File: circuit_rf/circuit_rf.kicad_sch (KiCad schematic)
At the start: 13 parts, among them J18 USB_C_Receptacle_USB2.0, U8 ESP32-C3, U9 SX1279, Y1 16M

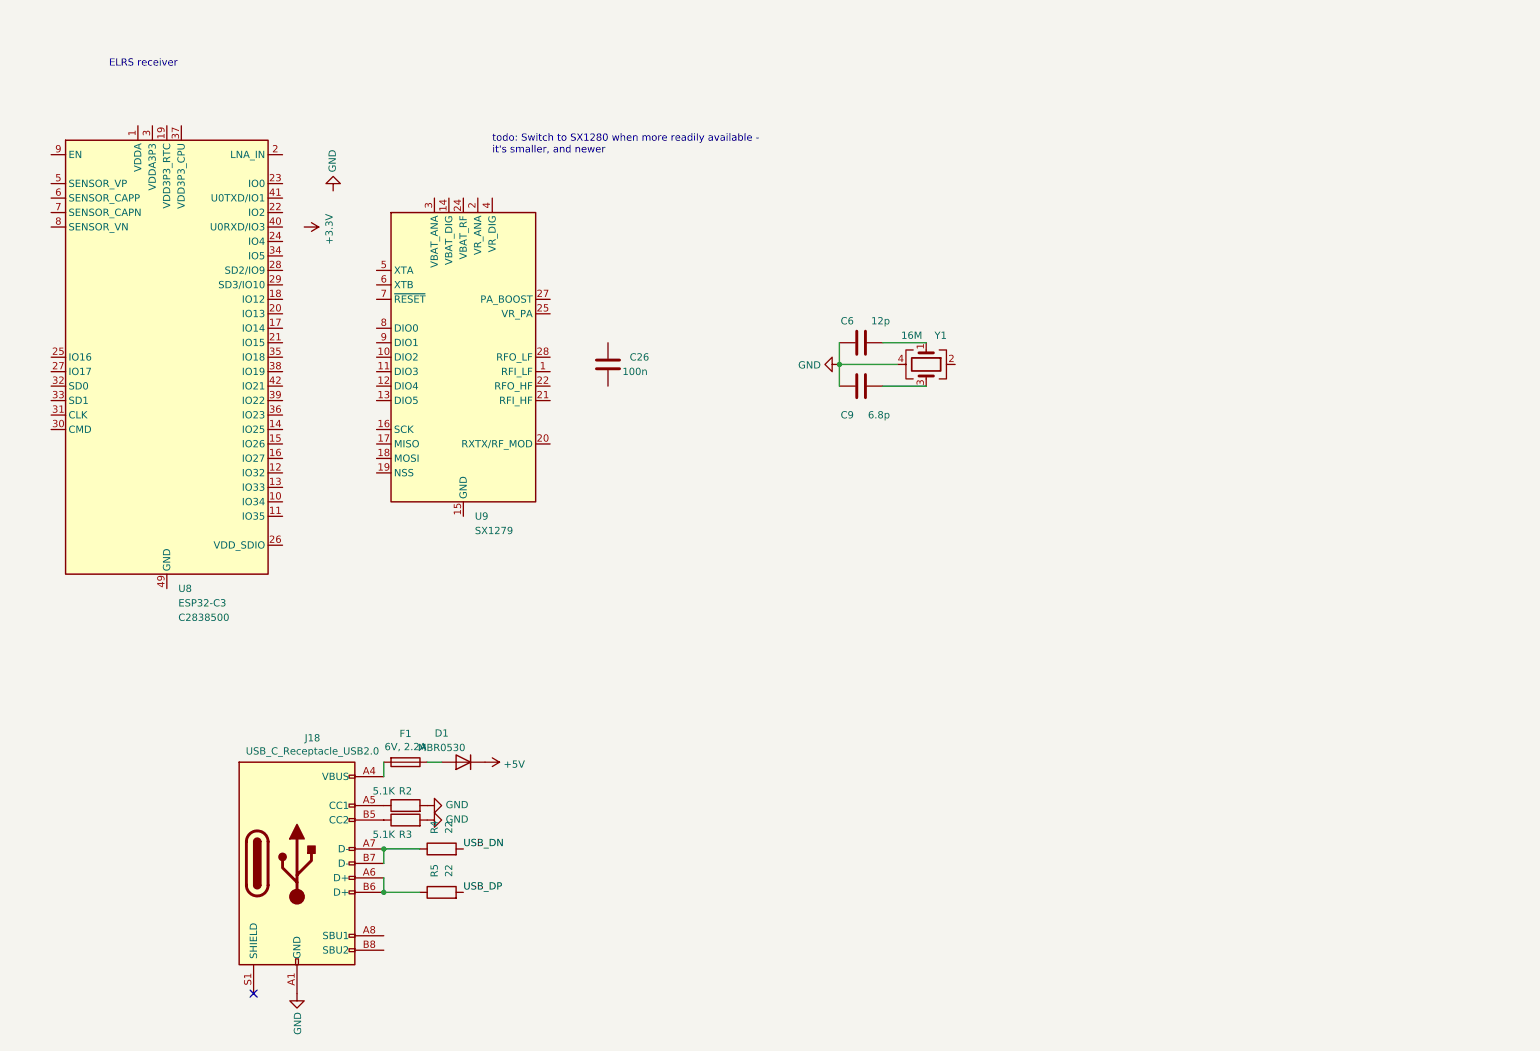
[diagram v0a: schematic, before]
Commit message: Lots of work on schematic, and BF cfg
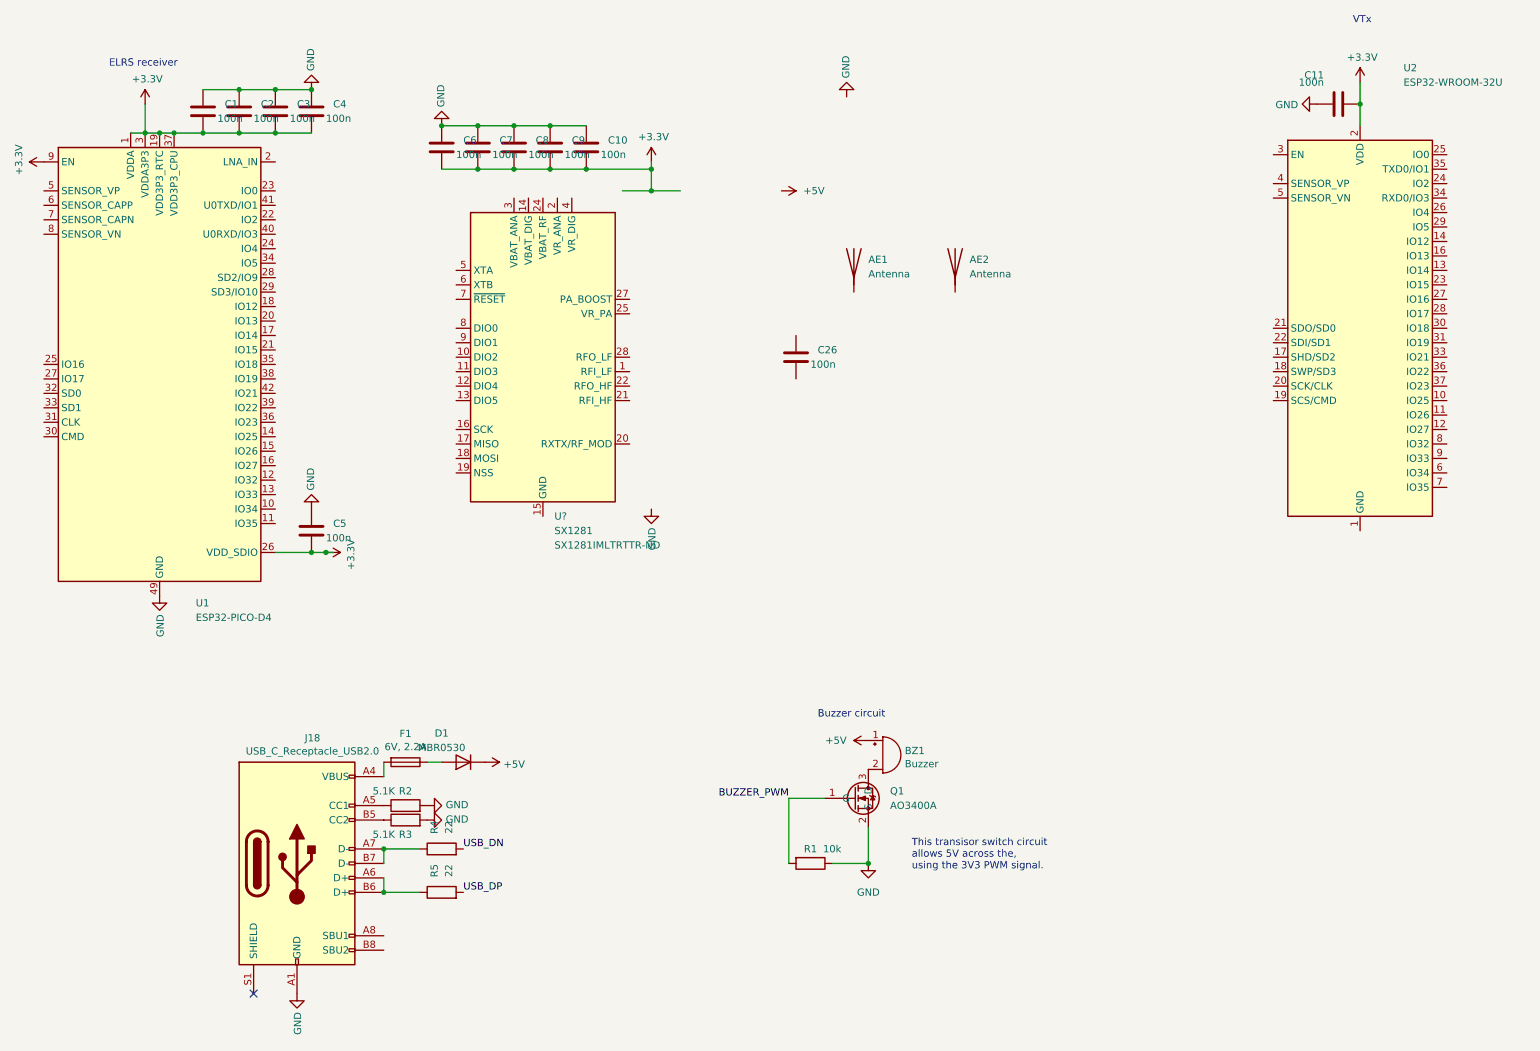
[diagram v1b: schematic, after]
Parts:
- removed U8: ESP32-C3, Package_DFN_QFN:QFN-32-1EP_5x5mm_P0.5mm_EP3.7x3.7mm, symbol Anyleaf_Shared:ESP32-C3
- removed U9: SX1279, Package_DFN_QFN:QFN-28-1EP_6x6mm_P0.65mm_EP4.8x4.8mm, symbol RF:SX1279
- removed Y1: 16M, Crystal:Crystal_SMD_2016-4Pin_2.0x1.6mm, symbol Device:Crystal_GND24
- added AE1, AE2: Antenna, symbol Device:Antenna
- added BZ1: Buzzer, Anyleaf_Shared:Buzzer_MLT-7525, symbol Device:Buzzer
- added C1, C10, C11, C2, C3, C4, C5, C7, C8: 100n, Capacitor_SMD:C_0402_1005Metric, symbol Device:C
- added Q1: AO3400A, Package_TO_SOT_SMD:SOT-23, symbol Anyleaf_Shared:AO3400A
- added R1: 10k, Resistor_SMD:R_0402_1005Metric, symbol Device:R
- added U1: ESP32-PICO-D4, Package_DFN_QFN:QFN-48-1EP_7x7mm_P0.5mm_EP5.3x5.3mm, symbol RF_Module:ESP32-PICO-D4
- added U2: ESP32-WROOM-32U, RF_Module:ESP32-WROOM-32U, symbol RF_Module:ESP32-WROOM-32U
- added U?: SX1281, Package_DFN_QFN:QFN-24-1EP_4x4mm_P0.5mm_EP2.6x2.6mm, symbol Anyleaf_Shared:SX1281
- C6: value 12p -> 100n; LCSC C1547 -> C1525
- C9: value 6.8p -> 100n; LCSC C1576 -> C1525
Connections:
- net +3V3: now also C6.2, C9.2, C1.2, C10.2, C11.2, C2.2, C3.2, C4.2, C5.2, C7.2, C8.2, U1.1 (VDDA), U1.19 (VDD3P3_RTC), U1.26 (VDD_SDIO), U1.3 (VDDA3P3), U1.37 (VDD3P3_CPU), U1.4 (VDDA3P3), U1.43 (VDDA), U1.46 (VDDA), U1.9 (EN), U2.2 (VDD)
- net +5V: now also BZ1.1 (-)
- net GND: now also C1.1, C10.1, C11.1, C2.1, C3.1, C4.1, C5.1, C7.1, C8.1, Q1.2 (S), R1.1, U1.49 (GND)
- new net: BZ1.2 (+), Q1.3 (D)
- new net: U2.1 (GND), U2.15 (GND), U2.38 (GND), U2.39 (GND)
- new net: U?.15 (GND), U?.23 (GND), U?.26 (GND), U?.29 (GND)
- new net BUZZER_PWM: Q1.1 (G), R1.2
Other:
- note added: "Buzzer circuit"
- note added: "This transisor switch circuit allows 5V across the, using the 3V3 PWM signal."
- note added: "VTx"
- note removed: "todo: Switch to SX1280 when more readily available - it's smaller, and newer"
- moved on the sheet: C26
